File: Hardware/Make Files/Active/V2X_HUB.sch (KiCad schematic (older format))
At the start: 13 parts, among them U20 USB2242, X3 24MHz

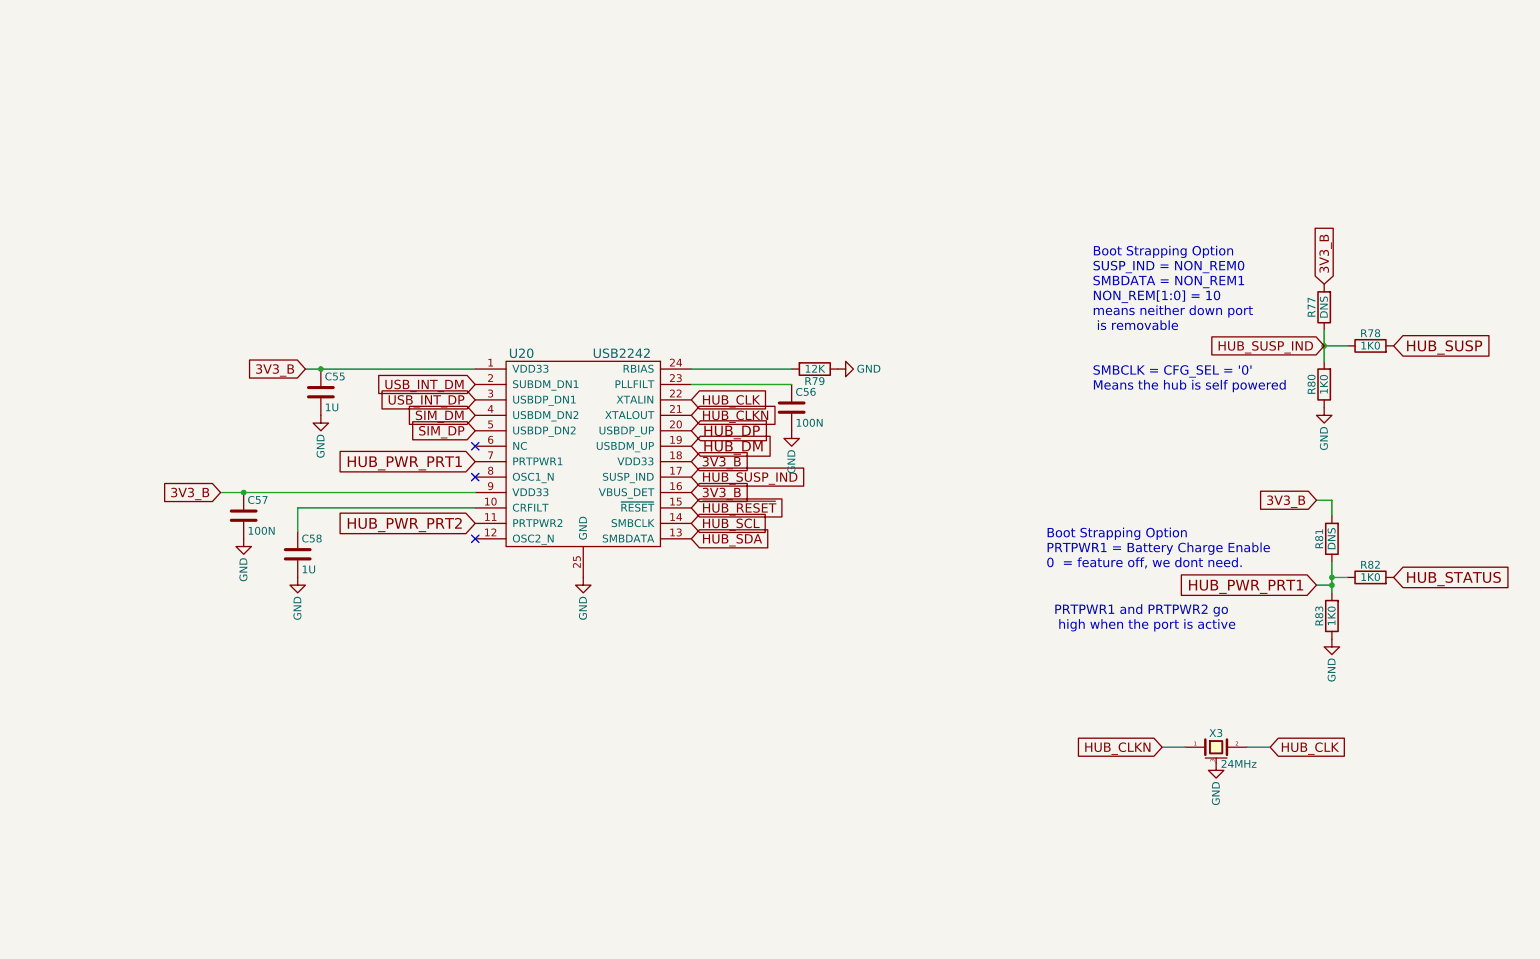
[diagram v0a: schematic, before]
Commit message: work from home day
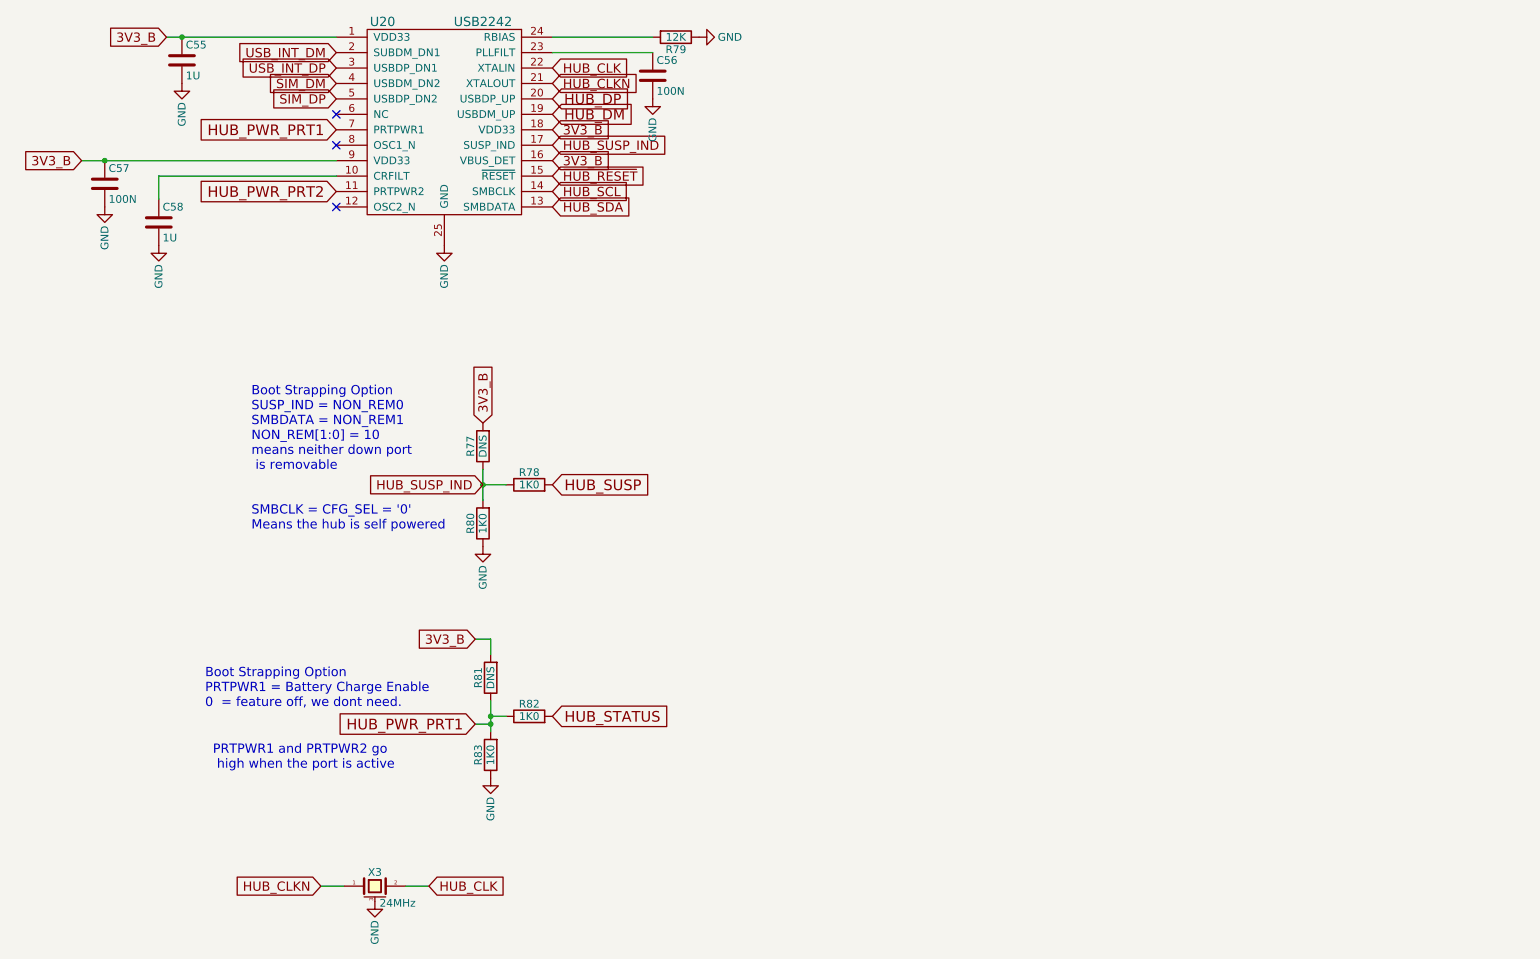
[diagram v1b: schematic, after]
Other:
- moved on the sheet: C55, C56, C57, C58, R77, R78, R79, R80, R81, R82, R83, U20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
